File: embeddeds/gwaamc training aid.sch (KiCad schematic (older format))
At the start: 19 parts, among them J1 Conn_Coaxial, U1 LM334Z, U2 LM334Z, U3-A , U3-B U3_AD8244ARMZ, U3-C U3_AD8244ARMZ, U3-D U3_AD8244ARMZ, U4 74LV138 only needed with larg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, U5... 74LV138 only for large number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

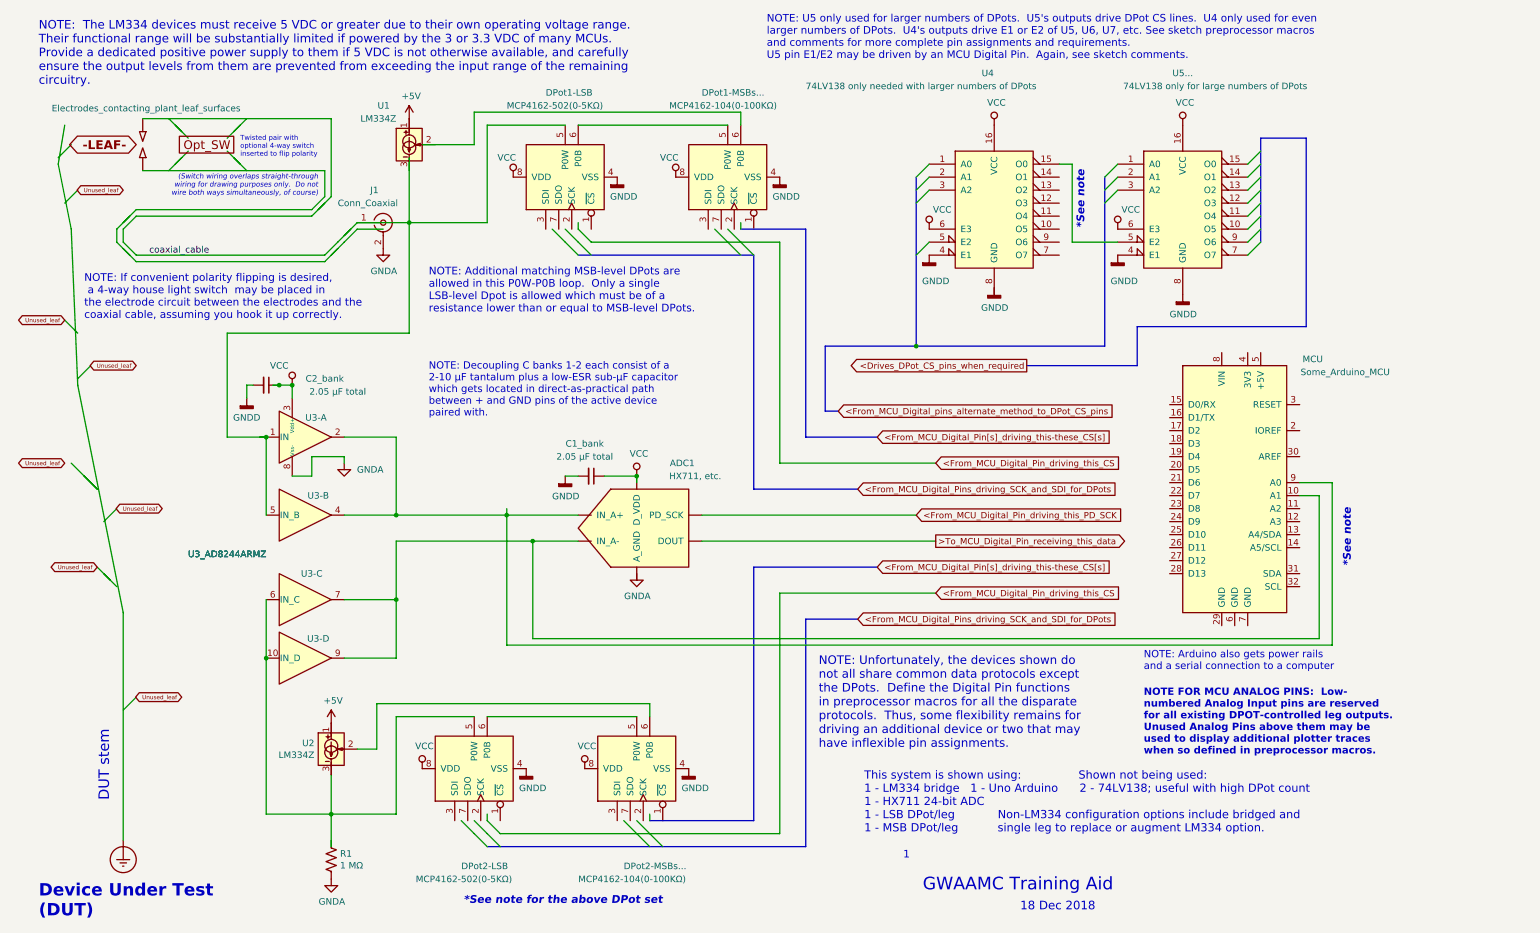
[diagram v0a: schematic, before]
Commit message: Add files via upload
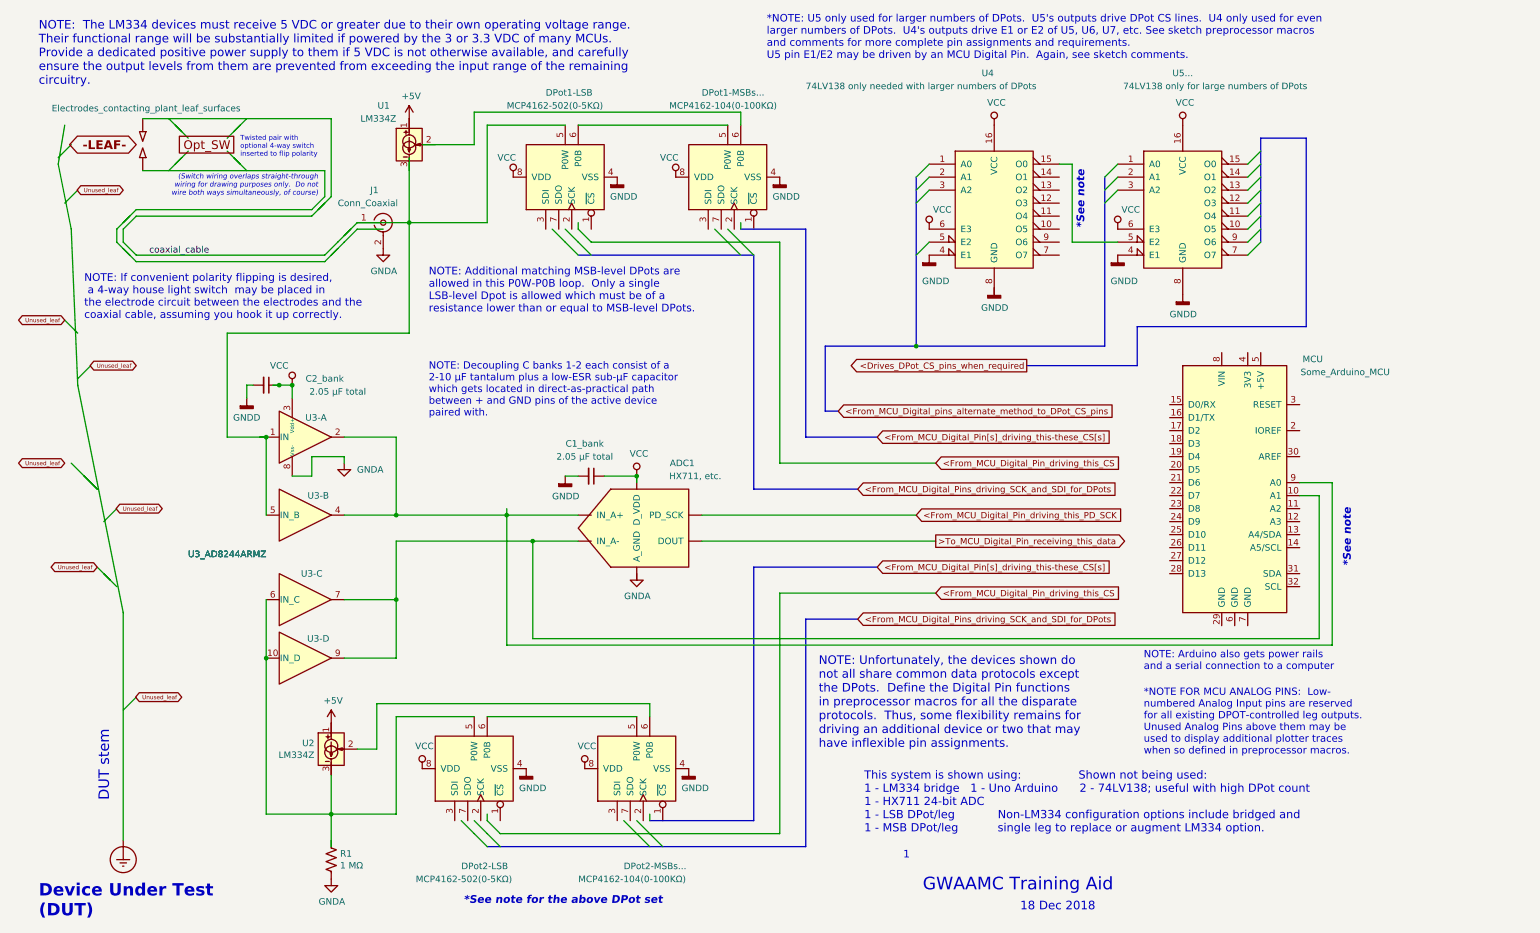
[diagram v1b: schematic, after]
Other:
- note added: "*NOTE FOR MCU ANALOG PINS: Low-\nnumbered Analog Input pins are reserved \nfor all existing DPOT-controlled leg outputs. \nUnused Analog Pins above them may be\nused to display additional plotter traces\nwhen so defined in preprocessor macros."
- note added: "*NOTE: U5 only used for larger numbers of DPots. U5's outputs drive DPot CS lines. U4 only used for even \nlarger numbers of DPots. U4's outputs drive E1 or E2 of U5, U6, U7, etc. See sketch preprocessor macros \nand comments for more complete pin assignments and requirements.\nU5 pin E1/E2 may be driven by an MCU Digital Pin. Again, see sketch comments."
- note removed: "NOTE FOR MCU ANALOG PINS: Low-\nnumbered Analog Input pins are reserved \nfor all existing DPOT-controlled leg outputs. \nUnused Analog Pins above them may be\nused to display additional plotter traces\nwhen so defined in preprocessor macros."
- note removed: "NOTE: U5 only used for larger numbers of DPots. U5's outputs drive DPot CS lines. U4 only used for even \nlarger numbers of DPots. U4's outputs drive E1 or E2 of U5, U6, U7, etc. See sketch preprocessor macros \nand comments for more complete pin assignments and requirements.\nU5 pin E1/E2 may be driven by an MCU Digital Pin. Again, see sketch comments."
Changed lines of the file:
@@
 $EndComp
 Text Notes 6250 1100 0    58   ~ 0
-NOTE: U5 only used for larger numbers of DPots.  U5's outputs drive DPot CS lines.  U4 only used for even \nlarger numbers of DPots.  U4's outputs drive E1 or E2 of U5, U6, U7, etc. See sketch preprocessor macros \nand comments for more complete pin assignments and requirements.\nU5 pin E1/E2 may be driven by an MCU Digital Pin.  Again, see sketch comments.
+*NOTE: U5 only used for larger numbers of DPots.  U5's outputs drive DPot CS lines.  U4 only used for even \nlarger numbers of DPots.  U4's outputs drive E1 or E2 of U5, U6, U7, etc. See sketch preprocessor macros \nand comments for more complete pin assignments and requirements.\nU5 pin E1/E2 may be driven by an MCU Digital Pin.  Again, see sketch comments.
 $Comp
 L power:GNDD #PWR?
@@
 Text Notes 10750 5000 1    60   Italic 12
 *See note
-Text Notes 9150 6450 0    56   ~ 11
-NOTE FOR MCU ANALOG PINS:  Low-\nnumbered Analog Input pins are reserved \nfor all existing DPOT-controlled leg outputs.  \nUnused Analog Pins above them may be\nused to display additional plotter traces\nwhen so defined in preprocessor macros.
+Text Notes 9150 6450 0    56   ~ 0
+*NOTE FOR MCU ANALOG PINS:  Low-\nnumbered Analog Input pins are reserved \nfor all existing DPOT-controlled leg outputs.  \nUnused Analog Pins above them may be\nused to display additional plotter traces\nwhen so defined in preprocessor macros.
 Text Notes 3650 3850 0    56   ~ 0
 NOTE: Decoupling C banks 1-2 each consist of a \n2-10 µF tantalum plus a low-ESR sub-µF capacitor \nwhich gets located in direct-as-practical path \nbetween + and GND pins of the active device \npaired with.
